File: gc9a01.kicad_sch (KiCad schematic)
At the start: 5 parts, among them J301 Conn_01x12_Pin, Q301 L2N7002SLLT1G

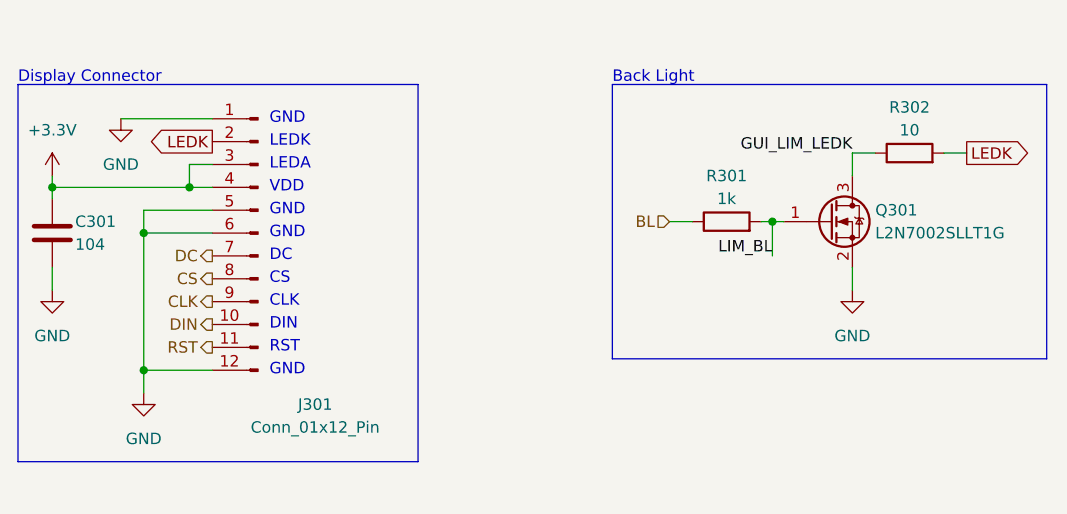
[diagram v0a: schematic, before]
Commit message: Finished v1.1
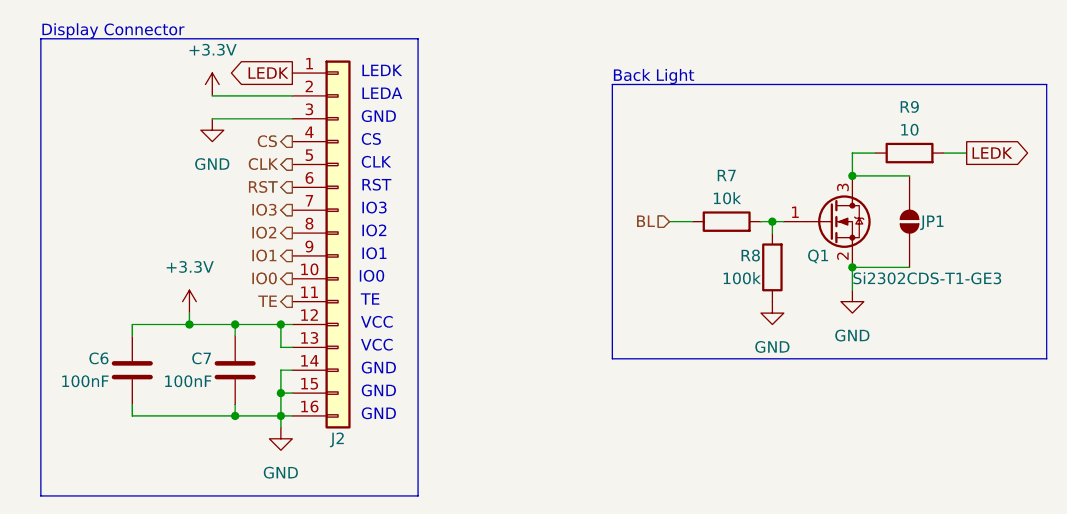
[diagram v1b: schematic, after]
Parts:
- removed J301: Conn_01x12_Pin, CustomFootprints:GC9A01_Connector, symbol Connector:Conn_01x12_Pin
- added C6: 100nF, Capacitor_SMD:C_0805_2012Metric, symbol Device:C
- added J2: Conn_01x16, CustomFootprints:ST77916, symbol Connector_Generic:Conn_01x16
- added JP1: SolderJumper_2_Open, Jumper:SolderJumper-2_P1.3mm_Open_Pad1.0x1.5mm, symbol Jumper:SolderJumper_2_Open
- added R8: 100k, Resistor_SMD:R_0603_1608Metric, symbol Device:R
- C7: renamed from C301; value 104 -> 100nF
- Q1: renamed from Q301; value L2N7002SLLT1G -> Si2302CDS-T1-GE3; footprint CustomFootprints:SOT_TO_92_L2N7002SLLT1G -> Package_TO_SOT_SMD:SOT-23
- R7: renamed from R301; value 1k -> 10k
- renumbered R302 to R9
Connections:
- net +3.3V: now also C6.1, J2.12 (Pin_12), J2.13 (Pin_13), J2.2 (Pin_2)
- net CLK: now also J2.5 (Pin_5)
- net CS: now also J2.4 (Pin_4)
- net GND: now also C6.2, J2.14 (Pin_14), J2.15 (Pin_15), J2.16 (Pin_16), J2.3 (Pin_3), JP1.2 (B), R8.1
- net LEDK: now also J2.1 (Pin_1)
- net RST: now also J2.6 (Pin_6)
- net GUI_LIM_LEDK: no longer names the net of Q1.3 (D), R9.1
- net GUI_LIM_LEDK: now also JP1.1 (A)
- net LIM_BL: no longer names the net of Q1.1 (G), R7.2
- net LIM_BL: now also R8.2
- new net IO0: J2.10 (Pin_10)
- new net IO1: J2.9 (Pin_9)
- new net IO2: J2.8 (Pin_8)
- new net IO3: J2.7 (Pin_7)
- new net TE: J2.11 (Pin_11)
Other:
- note added: "IO0"
- note added: "IO1"
- note added: "IO2"
- note added: "IO3"
- note added: "TE"
- note added: "VCC"
- note removed: "DC"
- note removed: "DIN"
- note removed: "VDD"
- moved on the sheet: C7
